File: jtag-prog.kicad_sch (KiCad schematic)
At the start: 40 parts, among them J14 USB_C_Receptacle_USB2.0_14P, J15 Conn_ST_STDC14, J20 Conn_01x10, U12 93LCxxA, U13 AMS1117-3.3, U14 FT2232HQ, Y2 12Mhz

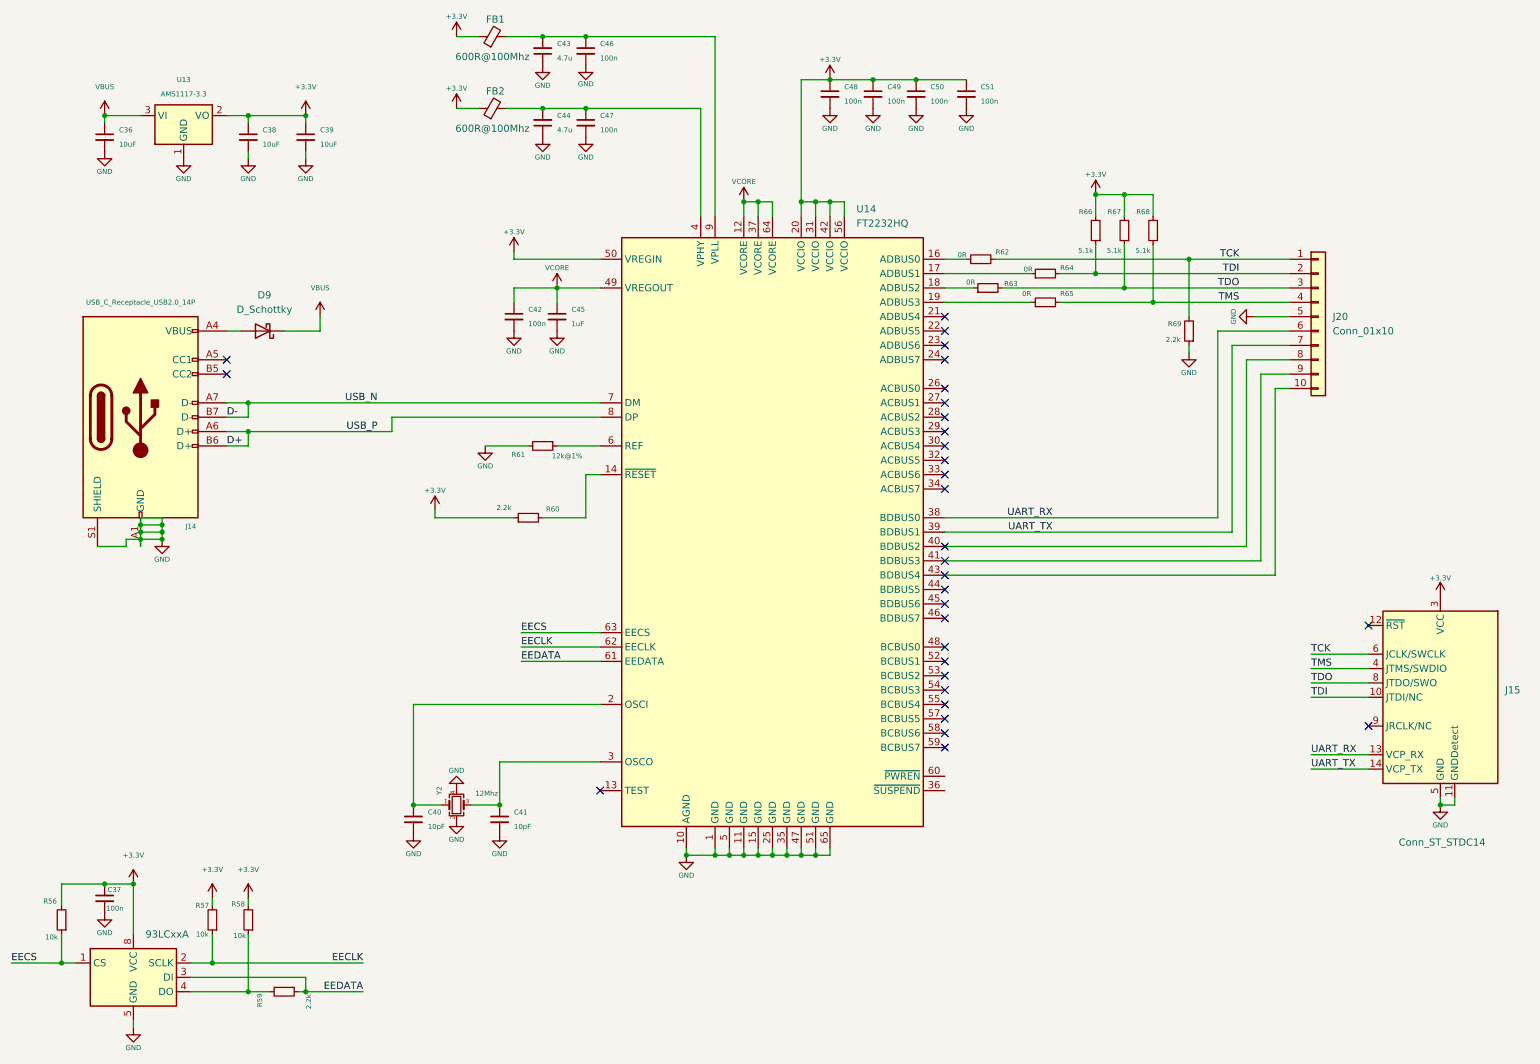
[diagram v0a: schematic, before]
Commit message: Update the source files
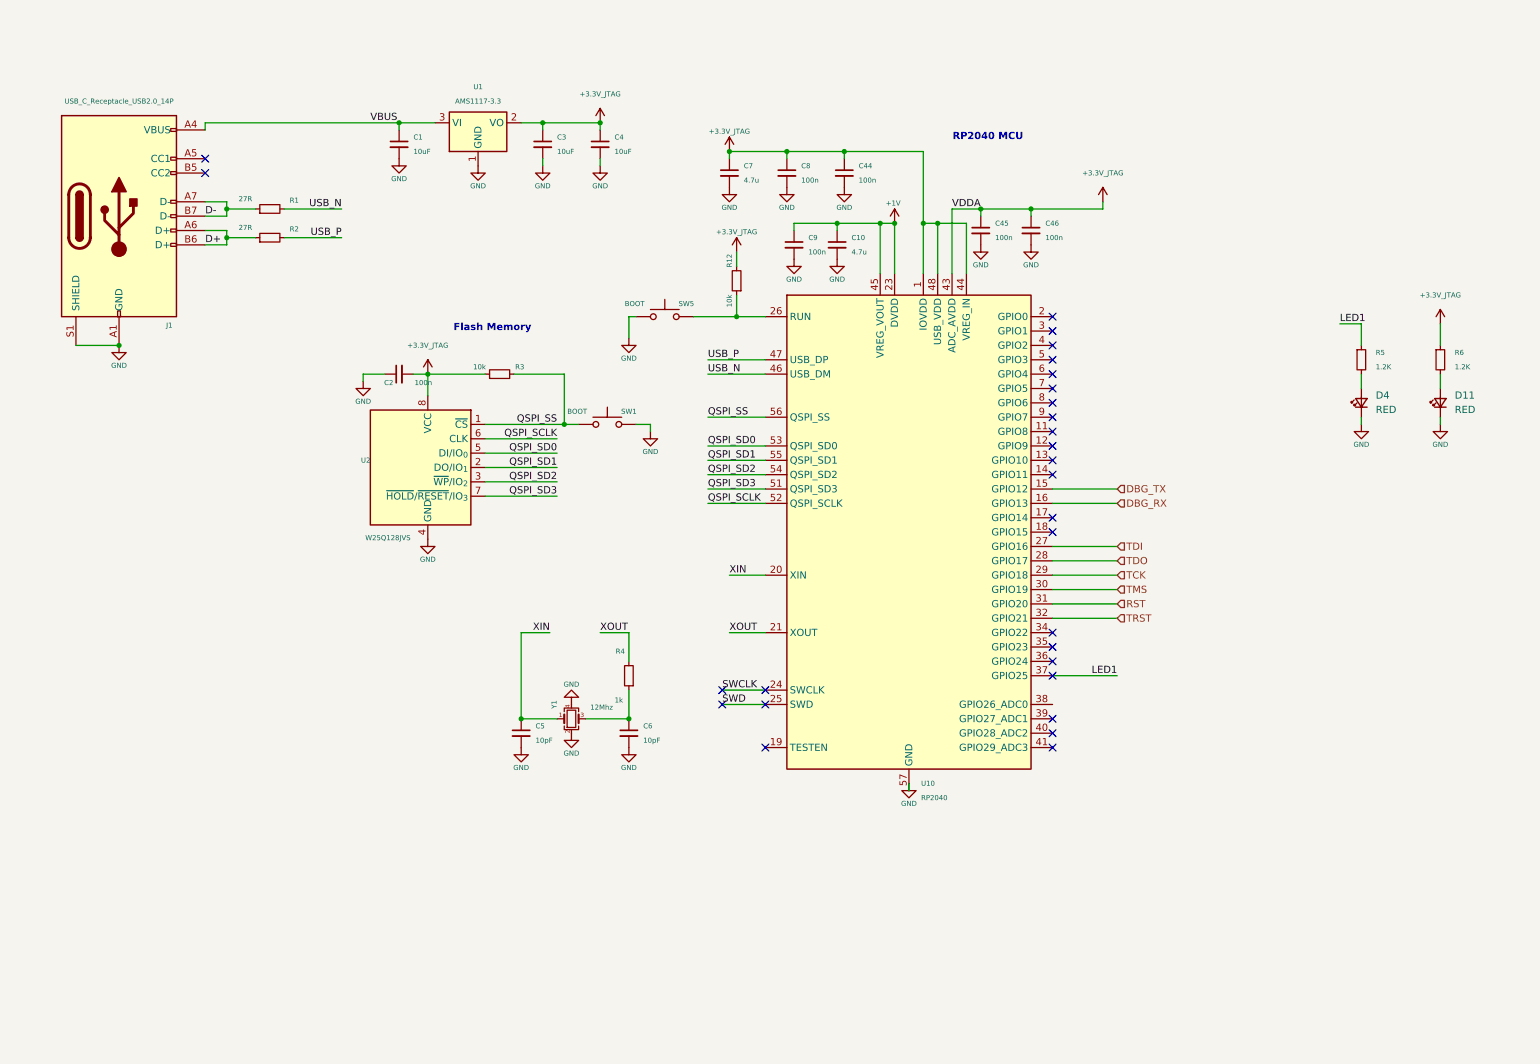
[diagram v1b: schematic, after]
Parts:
- removed C37, C42, C47, C48, C49, C50, C51: 100n, Capacitor_SMD:C_0402_1005Metric, symbol Device:C_Small
- removed C40, C41: 10pF, Capacitor_SMD:C_0402_1005Metric, symbol Device:C_Small
- removed C43: 4.7u, Capacitor_SMD:C_0603_1608Metric, symbol Device:C_Small
- removed D9: D_Schottky, Diode_SMD:D_SOD-123, symbol Device:D_Schottky
- removed FB1, FB2: 600R@100Mhz, Inductor_SMD:L_0603_1608Metric, symbol Device:FerriteBead_Small
- removed J14: USB_C_Receptacle_USB2.0_14P, Connector_USB:USB_C_Receptacle_G-Switch_GT-USB-7010ASV, symbol Connector:USB_C_Receptacle_USB2.0_14P
- removed J15: Conn_ST_STDC14, Connector_PinHeader_1.27mm:PinHeader_2x07_P1.27mm_Vertical, symbol Connector:Conn_ST_STDC14
- removed J20: Conn_01x10, Connector_PinHeader_2.54mm:PinHeader_1x10_P2.54mm_Vertical, symbol Connector_Generic:Conn_01x10
- removed R56, R57, R58: 10k, Resistor_SMD:R_0402_1005Metric, symbol Device:R_Small
- removed R59, R60, R69: 2.2k, Resistor_SMD:R_0402_1005Metric, symbol Device:R_Small
- removed R61: 12k@1%, Resistor_SMD:R_0402_1005Metric, symbol Device:R_Small
- removed R62, R63, R64, R65: 0R, Resistor_SMD:R_0402_1005Metric, symbol Device:R_Small
- removed R66, R67, R68: 5.1k, Resistor_SMD:R_0402_1005Metric, symbol Device:R_Small
- removed U12: 93LCxxA, Package_SO:SOIC-8_3.9x4.9mm_P1.27mm, symbol Memory_EEPROM:93LCxxA
- removed U14: FT2232HQ, Package_DFN_QFN:QFN-64-1EP_9x9mm_P0.5mm_EP4.35x4.35mm, symbol Interface_USB:FT2232HQ
- removed Y2: 12Mhz, Crystal:Crystal_SMD_3225-4Pin_3.2x2.5mm, symbol Device:Crystal_GND24_Small
- added C10, C7: 4.7u, Capacitor_SMD:C_0603_1608Metric, symbol Device:C_Small
- added C2, C8, C9: 100n, Capacitor_SMD:C_0402_1005Metric, symbol Device:C_Small
- added C5, C6: 10pF, Capacitor_SMD:C_0402_1005Metric, symbol Device:C_Small
- added D11, D4: RED, LED_SMD:LED_0603_1608Metric, symbol Device:LED_Small
- added J1: USB_C_Receptacle_USB2.0_14P, Connector_USB:USB_C_Receptacle_G-Switch_GT-USB-7010ASV, symbol Connector:USB_C_Receptacle_USB2.0_14P
- added R1, R2: 27R, Resistor_SMD:R_0402_1005Metric, symbol Device:R_Small
- added R12, R3: 10k, Resistor_SMD:R_0402_1005Metric, symbol Device:R_Small
- added R4: 1k, Resistor_SMD:R_0402_1005Metric, symbol Device:R_Small
- added R5, R6: 1.2K, Resistor_SMD:R_0402_1005Metric, symbol Device:R_Small
- added SW1, SW5: BOOT, EasyEDA_Lib:SW-SMD_L3.9-W3.0-P4.45, symbol Switch:SW_Push
- added U10: RP2040, Package_DFN_QFN:QFN-56-1EP_7x7mm_P0.4mm_EP3.2x3.2mm, symbol MCU_RaspberryPi:RP2040
- added U2: W25Q128JVS, Package_SO:SOIC-8_5.3x5.3mm_P1.27mm, symbol Memory_Flash:W25Q128JVS
- added Y1: 12Mhz, Crystal:Crystal_SMD_3225-4Pin_3.2x2.5mm, symbol Device:Crystal_GND24_Small
- C44: value 4.7u -> 100n; footprint Capacitor_SMD:C_0603_1608Metric -> Capacitor_SMD:C_0402_1005Metric
- C45: value 1uF -> 100n; footprint Capacitor_SMD:C_0603_1608Metric -> Capacitor_SMD:C_0402_1005Metric
- renumbered C36 to C1, C38 to C3, C39 to C4, U13 to U1
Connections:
- net +3.3V is gone; now on net +3.3V_JTAG: C3.1, C4.1, U1.2 (VO)
- net VCORE is gone; now on net +3.3V_JTAG: C45.1
- net D+: now also J1.A6 (D+), J1.B6 (D+), R2.1
- net D-: now also J1.A7 (D-), J1.B7 (D-), R1.1
- net GND: now also C44.2, C10.2, C2.1, C5.2, C6.2, C7.2, C8.2, C9.2, D11.1 (K), D4.1 (K), J1.A1 (GND), J1.A12 (GND), J1.B1 (GND), J1.B12 (GND), J1.S1 (SHIELD), SW1.2, SW5.1, U10.57 (GND), U2.4 (GND), Y1.2, Y1.4; no longer C44.1
- net TCK: now also U10.29 (GPIO18)
- net TDI: now also U10.27 (GPIO16)
- net TDO: now also U10.28 (GPIO17)
- net TMS: now also U10.30 (GPIO19)
- net VBUS: now also J1.A4 (VBUS), J1.A9 (VBUS), J1.B4 (VBUS), J1.B9 (VBUS)
- net +3.3V_JTAG: now reaches C46.1
- net +3.3V_JTAG: now also C44.1, C2.2, C7.1, C8.1, R12.2, R3.1, R6.1, U10.1 (IOVDD), U10.10 (IOVDD), U10.22 (IOVDD), U10.33 (IOVDD), U10.42 (IOVDD), U10.43 (ADC_AVDD), U10.44 (VREG_IN), U10.48 (USB_VDD), U10.49 (IOVDD), U2.8 (VCC)
- new net: D11.2 (A), R6.2
- new net: R12.1, SW5.2, U10.26 (RUN)
- new net: D4.2 (A), R5.2
- new net: C6.1, R4.1, Y1.3
- new net +1V: C10.1, C9.1, U10.23 (DVDD), U10.45 (VREG_VOUT), U10.50 (DVDD)
- new net DBG_RX: U10.16 (GPIO13)
- new net DBG_TX: U10.15 (GPIO12)
- new net LED1: R5.1, U10.37 (GPIO25)
- new net QSPI_SCLK: U10.52 (QSPI_SCLK), U2.6 (CLK)
- new net QSPI_SD0: U10.53 (QSPI_SD0), U2.5 (DI/IO_{0})
- new net QSPI_SD1: U10.55 (QSPI_SD1), U2.2 (DO/IO_{1})
- new net QSPI_SD2: U10.54 (QSPI_SD2), U2.3 (~{WP}/IO_{2})
- new net QSPI_SD3: U10.51 (QSPI_SD3), U2.7 (~{HOLD}/~{RESET}/IO_{3})
- new net QSPI_SS: R3.2, SW1.1, U10.56 (QSPI_SS), U2.1 (~{CS})
- new net RST: U10.31 (GPIO20)
- new net SWCLK: U10.24 (SWCLK)
- new net SWD: U10.25 (SWD)
- new net TRST: U10.32 (GPIO21)
- new net USB_N: R1.2, U10.46 (USB_DM)
- new net USB_P: R2.2, U10.47 (USB_DP)
- new net XIN: C5.1, U10.20 (XIN), Y1.1
- new net XOUT: R4.2, U10.21 (XOUT)
- no-connect marks 31 -> 28
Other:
- note added: "Flash Memory"
- note added: "RP2040 MCU"
- moved on the sheet: C1, C3, C4, U1
